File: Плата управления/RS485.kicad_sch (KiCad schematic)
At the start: 4 parts, among them U8 ADM3491ARZ

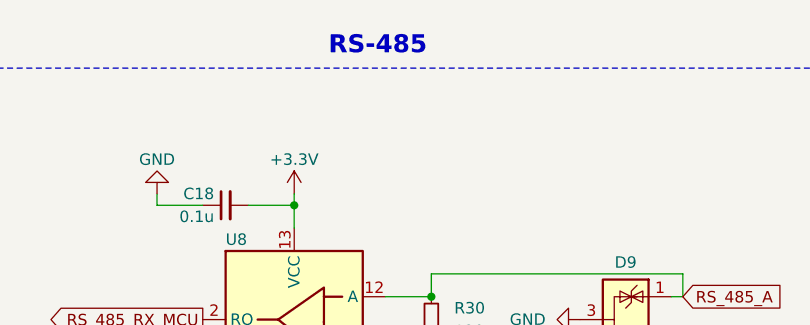
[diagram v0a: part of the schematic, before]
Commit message: Версия под отчёт
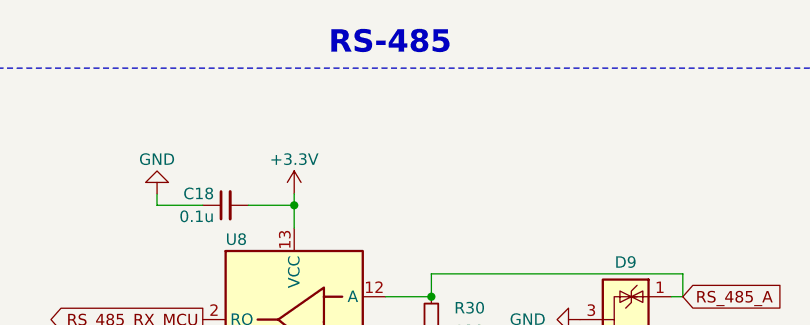
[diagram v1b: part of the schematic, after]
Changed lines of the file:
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@@
   )
   (text "RS-485" (at 153.67 64.77 0)
-    (effects (font (size 2 2) (thickness 0.4) bold) (justify left bottom))
+    (effects (font (size 2.5 2.5) (thickness 0.4) bold) (justify left bottom))
   )
   (global_label "RS_485_Enable_MCU" (shape input) (at 135.89 97.79 180) (fields_autoplaced)
